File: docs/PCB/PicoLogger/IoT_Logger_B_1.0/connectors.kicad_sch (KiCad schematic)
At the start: 9 parts, among them J3 USB-C, J4 Sensor, J5 LCD 16x2, J6 Additional, J7 SPI, J8 CON, J9 CAN, U7 TPD2EUSB30

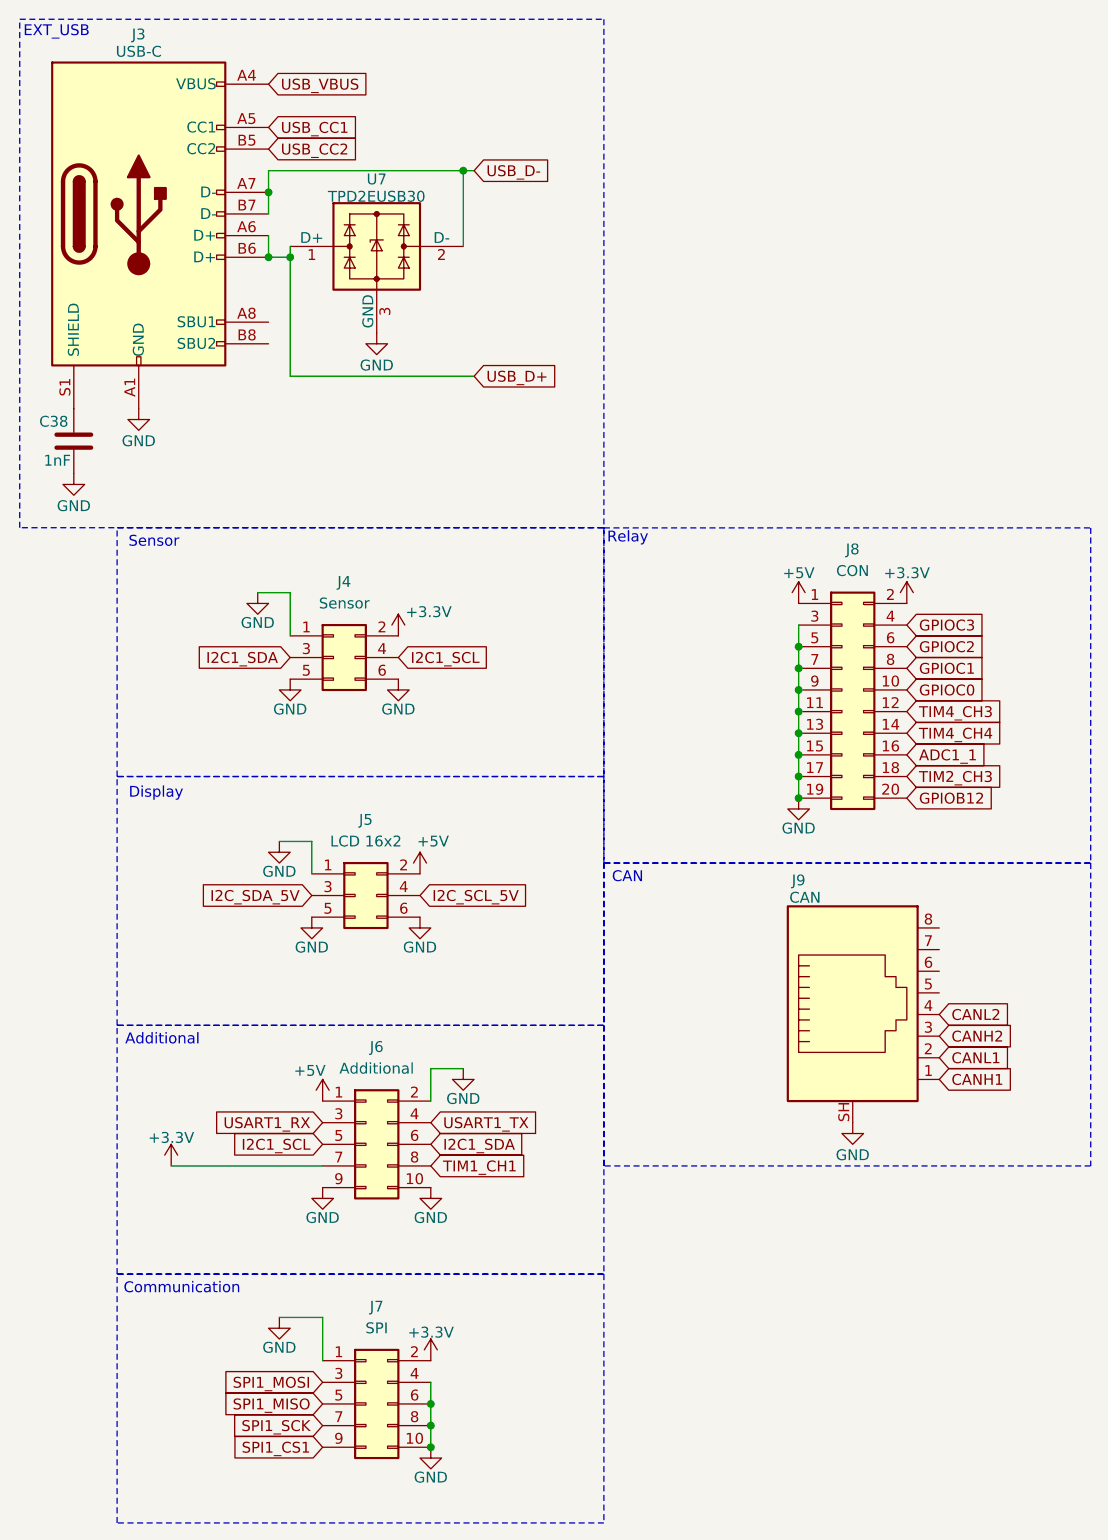
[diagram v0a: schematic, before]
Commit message: Code added, documentation review.
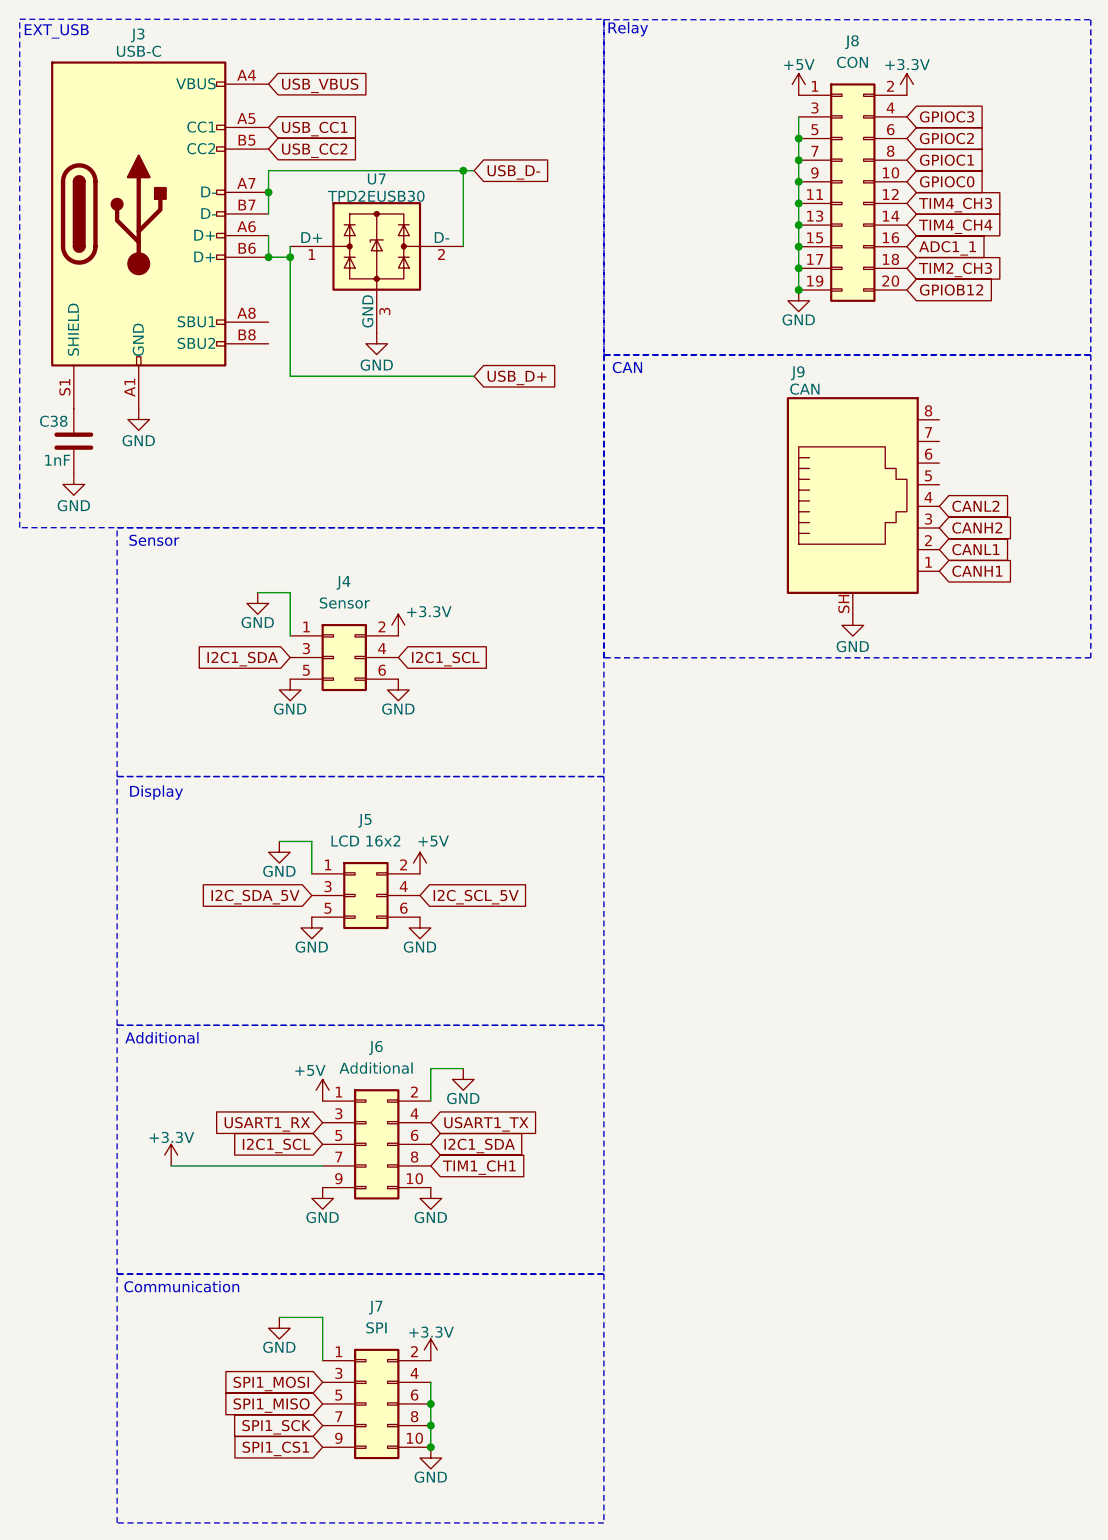
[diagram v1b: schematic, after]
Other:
- moved on the sheet: J8, J9
